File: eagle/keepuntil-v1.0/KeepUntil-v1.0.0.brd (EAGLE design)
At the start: 32 x 39 mm, 16 parts, among them IC2 REG1117, J1 USB-MICROB, Q1 CSTCR6M00G53Z, T1 BC846, U1 ATMEGA328P-AU

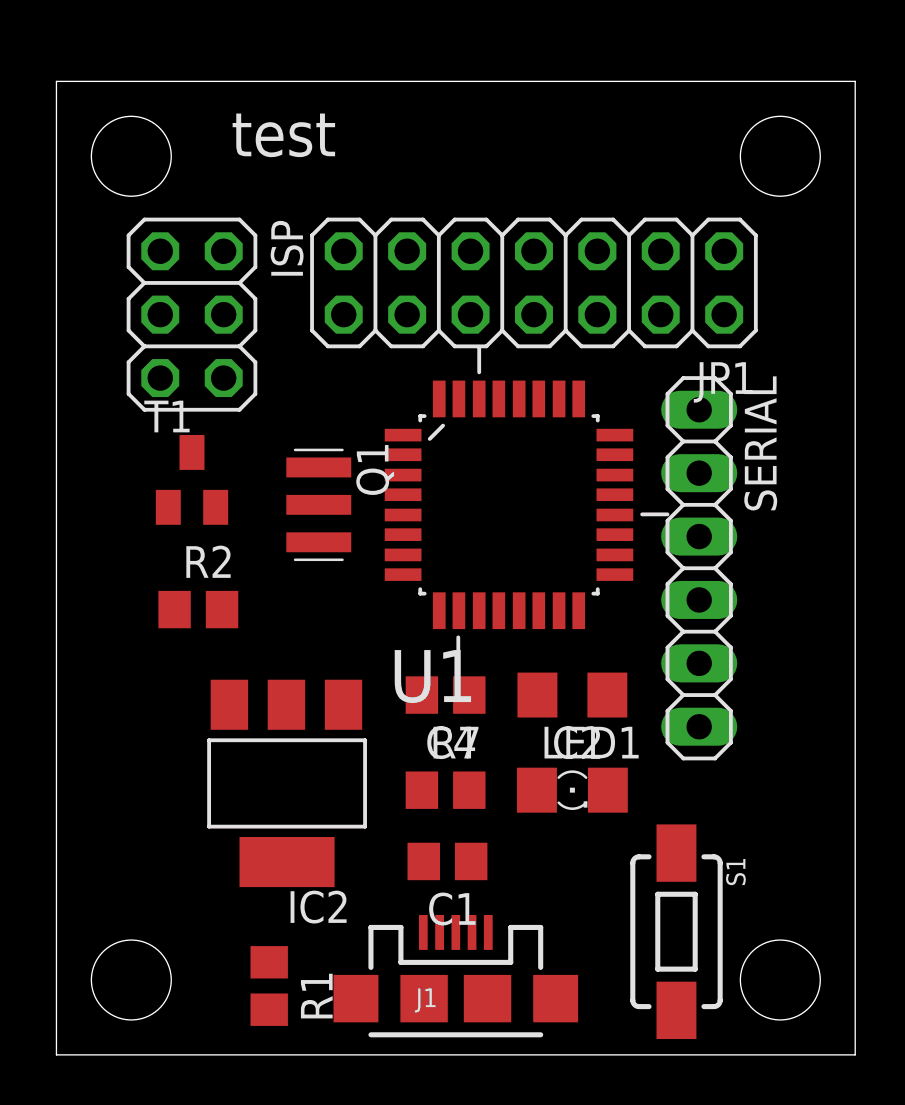
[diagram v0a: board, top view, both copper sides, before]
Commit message: board
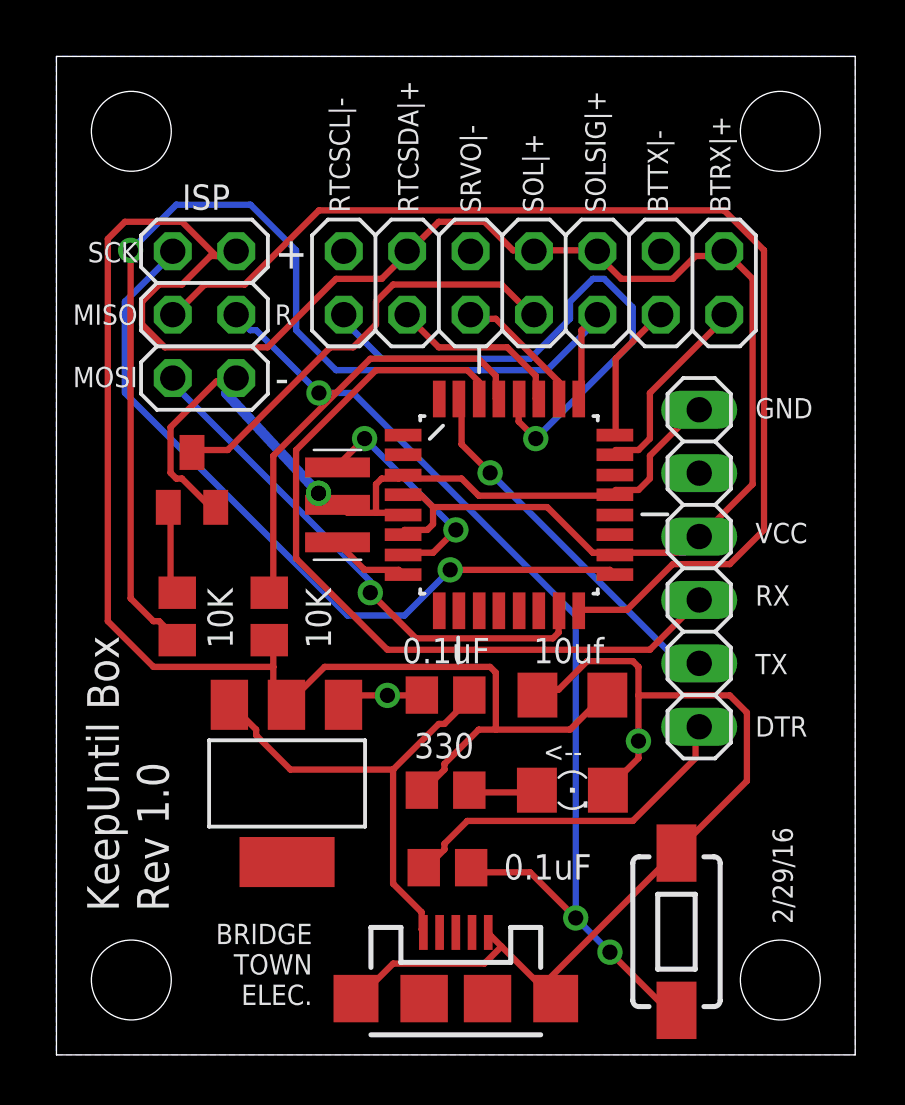
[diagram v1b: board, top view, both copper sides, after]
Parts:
- moved R1 14.8 mm to (8.53, 17.6)
- moved R2 0.89 mm to (4.84, 17.6), turned to 270 degrees
- moved Q1 0.75 mm to (11.3, 22.0)
- moved ISP 0.50 mm to (5.93, 29.7)
- moved C1 0.25 mm to (15.7, 7.50)
- turned R7 to 180 degrees
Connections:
- net SOLENOID-SIG: no longer U1.32
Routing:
- net VCC: track 0.00 -> 112.3 mm
- net GND: track 0.00 -> 78.3 mm, vias 0 -> 3
- net RESET: track 0.00 -> 59.7 mm, vias 0 -> 3
- net MISO: track 0.00 -> 46.0 mm
- net SOLENOID-SIG: track 0.00 -> 45.4 mm, vias 0 -> 1
- net RX: track 0.00 -> 32.4 mm
- net SCK: track 0.00 -> 30.6 mm, vias 0 -> 1
- net RTC-SCL: track 0.00 -> 23.4 mm, vias 0 -> 1
- net MOSI: track 0.00 -> 21.2 mm, vias 0 -> 1
- net N$4: track 0.00 -> 19.3 mm
- net SOLENOID: track 0.00 -> 17.5 mm
- net TX: track 0.00 -> 15.0 mm, vias 0 -> 1
- net N$17: track 0.00 -> 14.2 mm
- net N$1: track 0.00 -> 9.39 mm, vias 0 -> 2
- net BT-RX: track 0.00 -> 7.95 mm
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- added copper zone on layer 16, net GND
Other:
- board size 32 x 39 mm -> 32 x 40 mm
- board text added: "+"
- board text added: "-"
- board text added: "2/29/16"
- board text added: "<--"
- board text added: "BRIDGE TOWN ELEC."
- board text added: "BTRX|+"
- board text added: "BTTX|-"
- board text added: "DTR"
- board text added: "GND"
- board text added: "KeepUntil Box"
- board text added: "MISO"
- board text added: "MOSI"
- board text added: "R"
- board text added: "RTCSCL|-"
- board text added: "RTCSDA|+"
- board text added: "RX"
- board text added: "Rev 1.0"
- board text added: "SCK"
- board text added: "SOLSIG|+"
- board text added: "SOL|+"
- board text added: "SRVO|-"
- board text added: "TX"
- board text added: "VCC"
- board text removed: "test"
